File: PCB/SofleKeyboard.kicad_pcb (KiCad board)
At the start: 2 copper layers, 85 parts, among them J1 LED, J2 4PIN, J3 OLED, P1 i2c_pin, P2 i2c_pin, SW1 SW_PUSH, SW10 SW_PUSH, SW11 SW_PUSH, SW12 SW_PUSH, SW13 SW_PUSH, SW14 SW_PUSH, SW15 SW_PUSH, SW16 SW_PUSH, SW17 SW_PUSH, SW18 SW_PUSH, SW19 SW_PUSH, SW2 SW_PUSH, SW20 SW_PUSH, SW21 SW_PUSH, SW22 SW_PUSH, SW23 SW_PUSH, SW24 SW_PUSH, SW25 Rotary_Encoder_Switch, SW26 SW_PUSH, SW27 SW_PUSH, SW28 SW_PUSH, SW29 SW_PUSH, SW3 SW_PUSH, SW30 SW_PUSH, SW4 SW_PUSH, SW5 SW_PUSH, SW6 SW_PUSH, SW7 SW_PUSH, SW8 SW_PUSH, SW9 SW_PUSH, U1 ProMicro

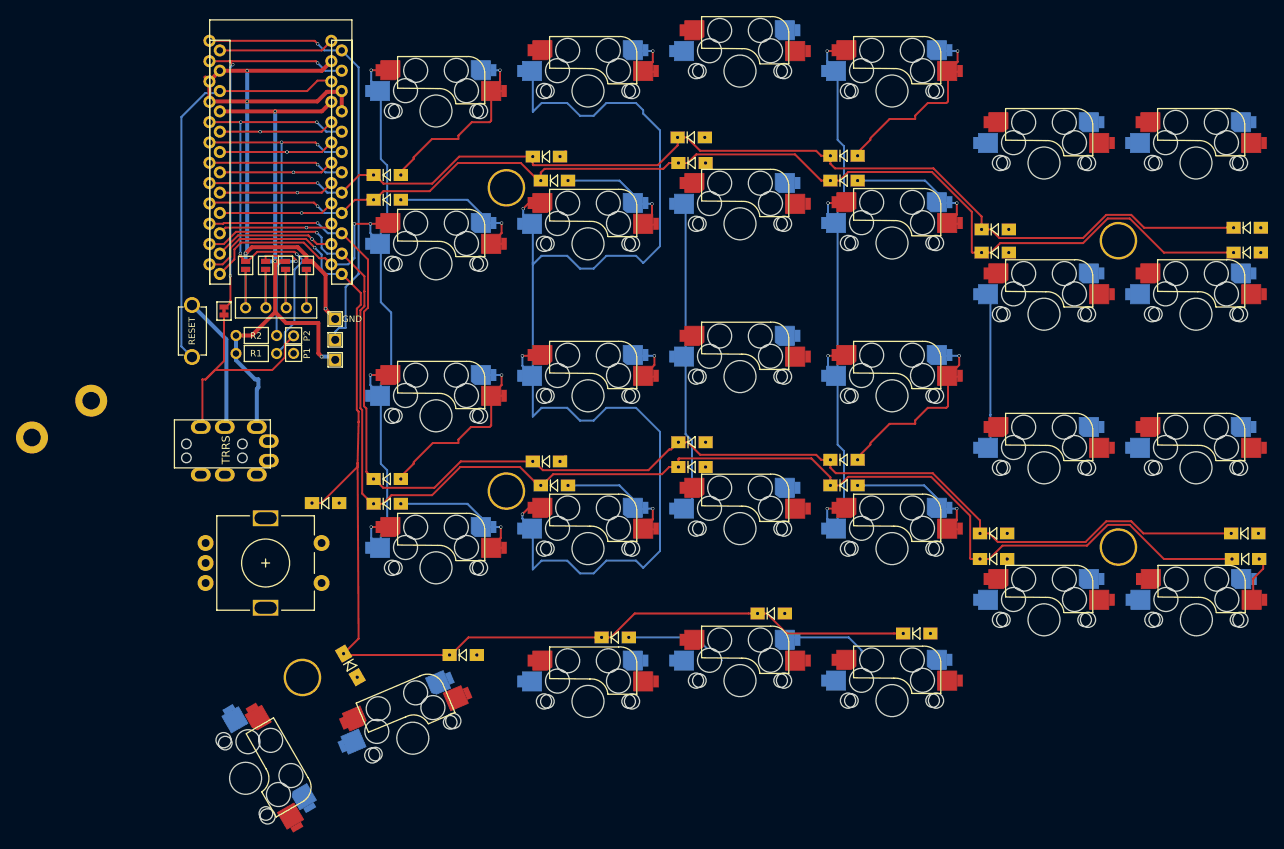
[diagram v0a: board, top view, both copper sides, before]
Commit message: WIP routing micro
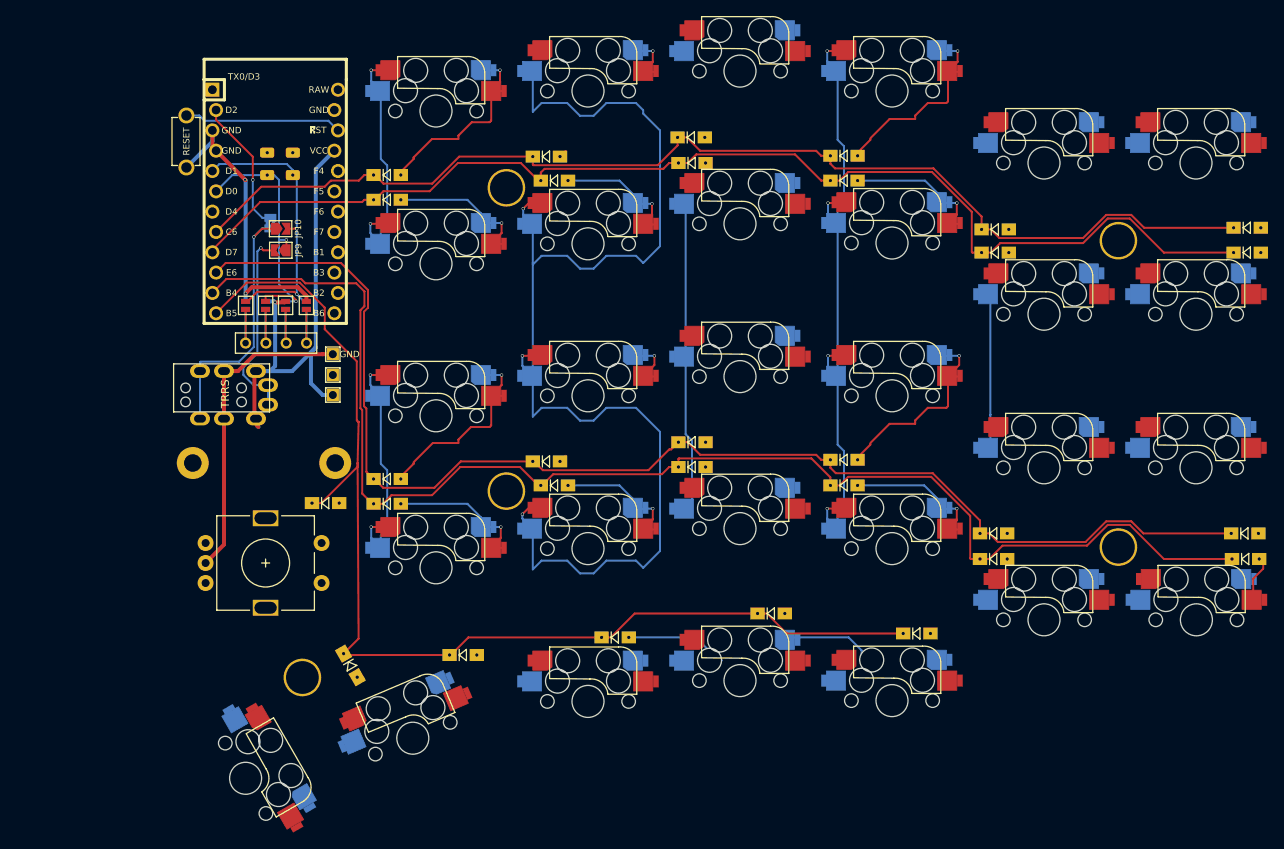
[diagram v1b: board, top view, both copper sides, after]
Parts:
- removed P1, P2: i2c_pin, SofleKeyboard-footprint:1pin_conn
- removed W1: jumper, SofleKeyboard-footprint:jumper_data
- added JP10: IC2SDA, Jumper:SolderJumper-2_P1.3mm_Open_TrianglePad1.0x1.5mm, F.Cu at (101.1, 64.7)
- added JP11: Serial, Jumper:SolderJumper-2_P1.3mm_Bridged2Bar_Pad1.0x1.5mm, B.Cu at (99.8, 64.0)
- added JP9: I2CSCL, Jumper:SolderJumper-2_P1.3mm_Open_TrianglePad1.0x1.5mm, F.Cu at (101.1, 67.4)
- R1, R2: footprint SofleKeyboard-footprint:RESISTOR_mini -> SofleKeyboard-footprint:R_1206_DoubleSided; moved to B.Cu
- U1: footprint SofleKeyboard-footprint:ProMicro -> Keebio:ArduinoProMicro-ZigZag
- moved TH2 31.3 mm to (107.9, 93.4)
- moved R1 24.1 mm to (102.6, 56.6), turned to 270 degrees
- moved RSW1 23.7 mm to (89.3, 53.8), turned to 90 degrees
- moved R2 21.5 mm to (99.4, 56.6), turned to 270 degrees
- moved TH1 20.4 mm to (90.1, 94.0)
- moved J2 7.00 mm to (87.7, 84.6)
- moved U1 5.34 mm to (100.4, 61.3), turned to 270 degrees
- moved JP1 5.00 mm to (104.3, 74.3)
- moved JP2 5.00 mm to (101.7, 74.3)
- moved JP3 5.00 mm to (99.2, 74.3)
- moved JP4 5.00 mm to (96.7, 74.3)
- moved JP5 5.00 mm to (104.3, 74.3)
- moved JP6 5.00 mm to (101.7, 74.3)
- moved JP7 5.00 mm to (99.2, 74.3)
- moved JP8 5.00 mm to (96.7, 74.3)
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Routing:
- net LED: track 55.8 -> 0.00 mm, vias 1 -> 0
- net SW25A: track 115.4 -> 68.4 mm, vias 5 -> 4
- net DATA: track 48.8 -> 16.9 mm, vias 3 -> 1
- net RESET: track 51.2 -> 19.7 mm
- net /i2c_c: track 0.57 -> 24.7 mm, vias 0 -> 1
- net GND: track 99.5 -> 78.1 mm, vias 4 -> 2
- net SDA: track 57.0 -> 36.0 mm, vias 4 -> 2
- net Net-(U1-Pad7): track 17.0 -> 0.00 mm, vias 1 -> 0
- net SCL: track 50.1 -> 33.5 mm, vias 3 -> 2
- net col4: track 181.0 -> 165.7 mm, vias 4 -> 3
- net col0: track 14.5 -> 0.00 mm, vias 1 -> 0
- net col1: track 33.7 -> 19.3 mm, vias 1 -> 0
- net col2: track 102.0 -> 87.5 mm, vias 5 -> 4
- net col3: track 50.6 -> 36.1 mm, vias 1 -> 0
- net Net-(U1-Pad24): track 14.4 -> 0.00 mm
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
